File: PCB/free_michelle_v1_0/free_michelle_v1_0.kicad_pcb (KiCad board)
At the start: 2 copper layers, 101 parts, among them J1 Zworka_TX, J10 ARK, J11 ARK, J12 Zworka_Buzzer, J13 ARK, J14 ARK, J15 Gniazdo 5VP DC 5,5x2,5, J16 Gniazdo 9V DC 5,5x2,5, J2 Zworka_RX, J3 GROVE_SW, J4 ARK, J5 ARK, J6 ARK, J7 ARK, J8 GROVE_SW, J9 A02YYUW_GroveCON, K1 FINDER-36.11, K2 FINDER-36.11, K3 FINDER-36.11, K4 FINDER-36.11, K5 FINDER-36.11, K6 FINDER-36.11, K7 FINDER-36.11, K8 FINDER-36.11, Q1 MMBT4403_PNP, Q2 MMBT4403_PNP, Q3 MMBT4403_PNP, Q4 MMBT4403_PNP, Q5 BSS138, Q6 MMBT4403_PNP, Q7 MMBT4403_PNP, Q8 MMBT4403_PNP, Q9 MMBT4403_PNP, SW1 Rotary_Encoder, SW2 SW_Push, SW3 SW_Push, U1 EEPROM_24AA01, U2 ESP8266_NodeMCU_v2, U3 DS3231M_RTC, U4 NRF24L01_Breakout, U5 BMP280, U6 LD1117V33, U7 L7805, U8 LD1117V33

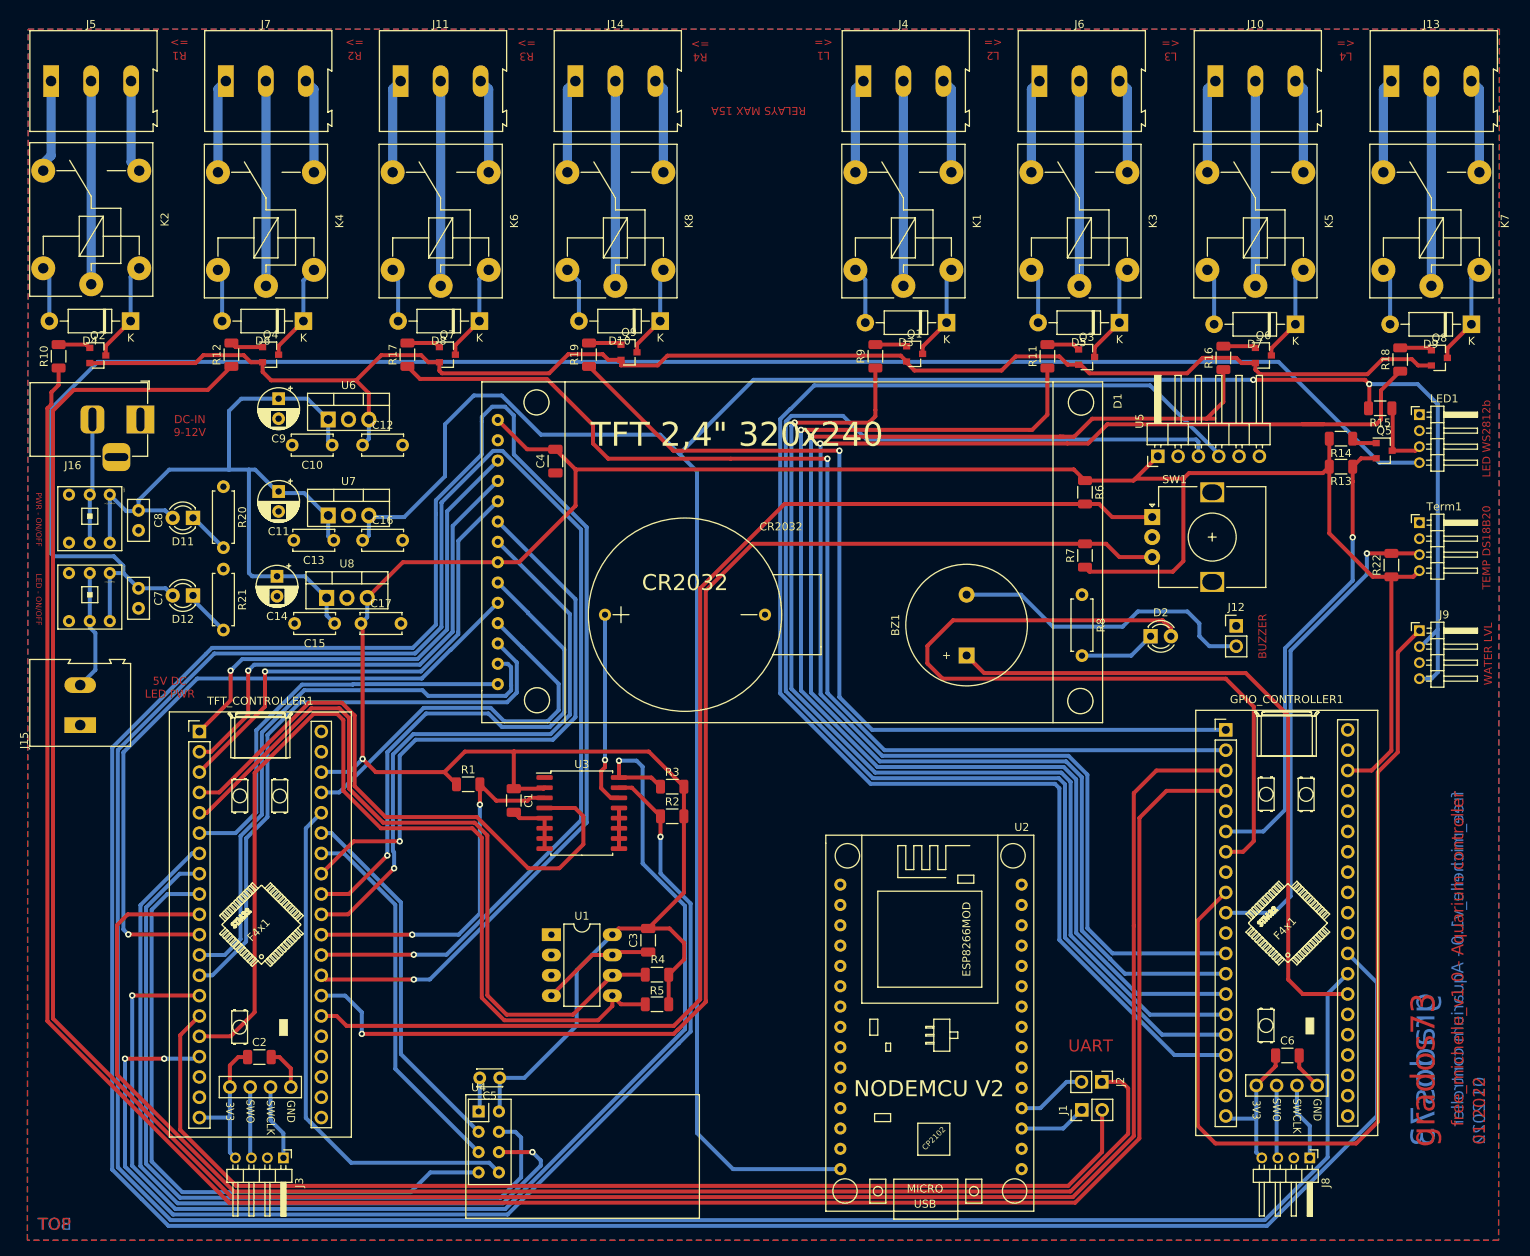
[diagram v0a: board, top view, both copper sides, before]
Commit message: Gotowa płytka przed generacją gerberow
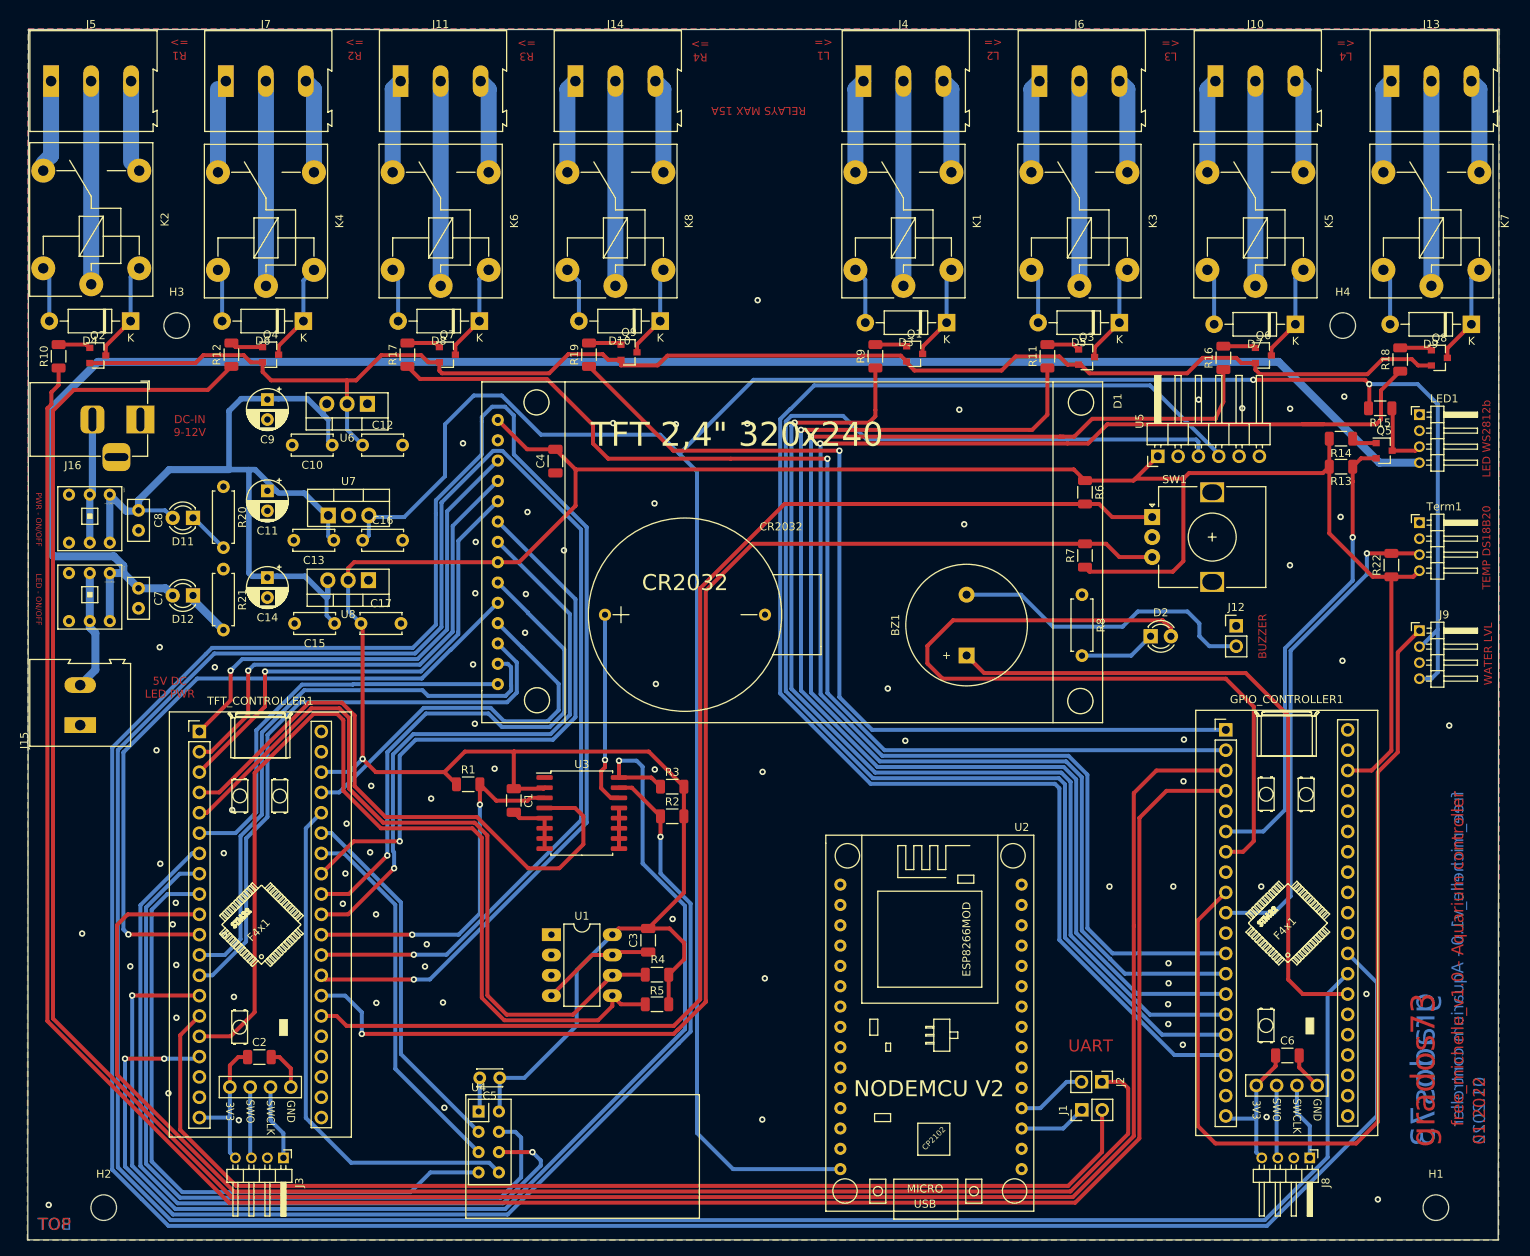
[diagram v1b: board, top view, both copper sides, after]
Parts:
- added H1: MountingHole, MountingHole:MountingHole_3.2mm_M3, F.Cu at (201.1, 163.0)
- added H2: MountingHole, MountingHole:MountingHole_3.2mm_M3, F.Cu at (34.5, 163.0)
- added H3: MountingHole, MountingHole:MountingHole_3.2mm_M3, F.Cu at (43.7, 52.8)
- added H4: MountingHole, MountingHole:MountingHole_3.2mm_M3, F.Cu at (189.4, 52.8)
- U6, U8: value LD1117V33 -> LD1117AV33
- moved U8 5.68 mm to (67.6, 84.6), turned to 180 degrees
- moved U6 5.28 mm to (67.5, 62.5), turned to 180 degrees
- moved C9 1.40 mm to (55.0, 62.0)
- moved C11 1.40 mm to (55.0, 73.4)
- moved C14 1.21 mm to (55.0, 84.3)
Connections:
- U6 pad 1: +9V -> GND
- U6 pad 2: GND -> +3.3VP
- U6 pad 3: +3.3VP -> +9V
- U8 pad 1: +9V -> GND
- U8 pad 2: GND -> +3V3
- U8 pad 3: +3V3 -> +9V
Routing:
- net +9V: track 99.9 -> 105.0 mm
- net +3V3: track 409.8 -> 414.7 mm
- net LIGHT3_PB5: track 168.5 -> 167.9 mm
- net GND: vias 4 -> 79
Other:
- board outline added: 183.9 x 151.3 mm
